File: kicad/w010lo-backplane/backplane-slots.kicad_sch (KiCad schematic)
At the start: 8 parts, among them J3 VME, J4 VME, J5 VME, J6 VME

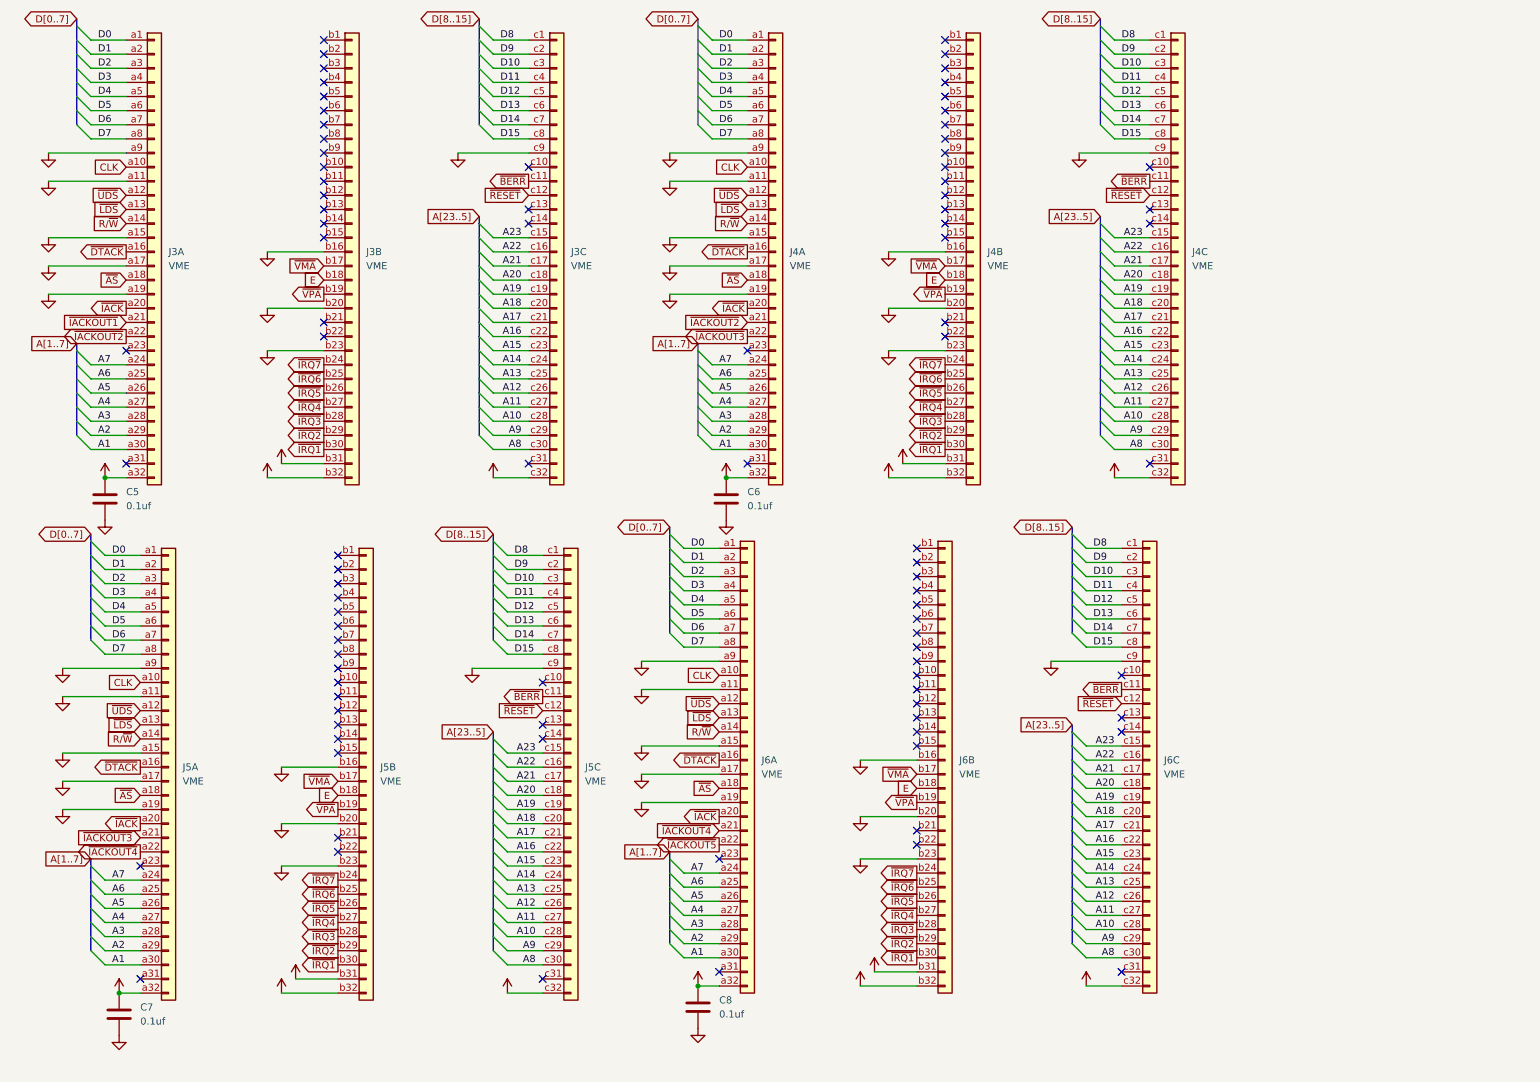
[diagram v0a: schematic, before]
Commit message: Final Kicad update before manufacturing
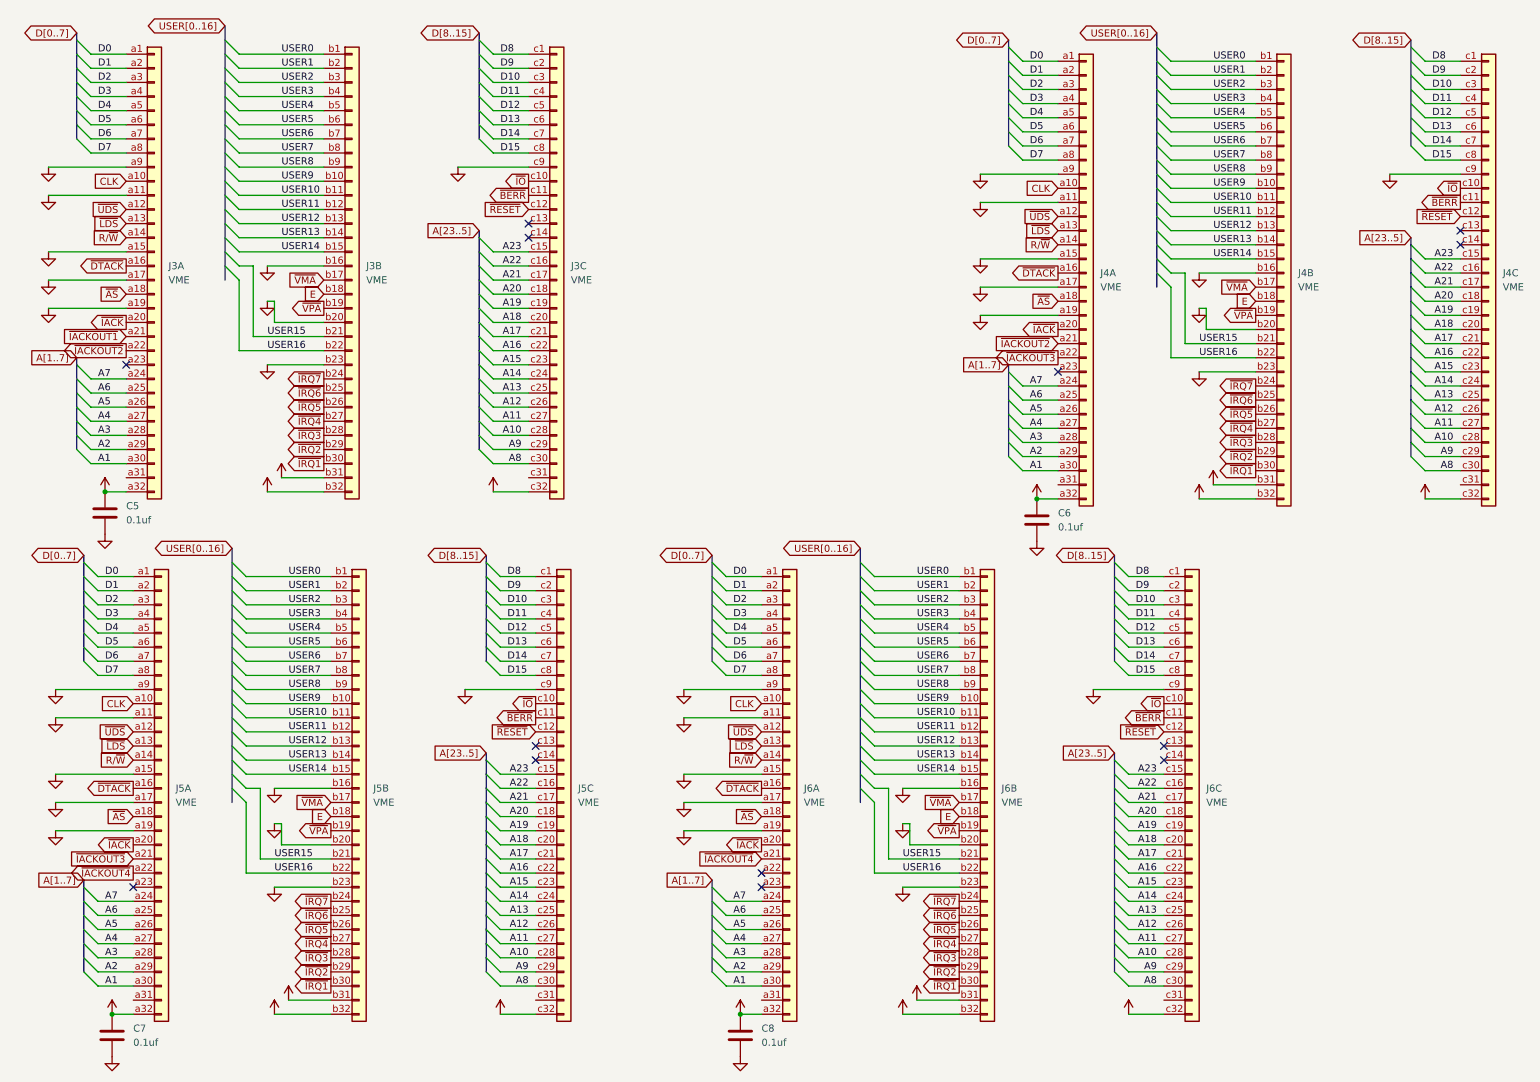
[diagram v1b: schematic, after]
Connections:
- net ~{IO}: now reaches J6.c10 (Pin_c10)
- net ~{IO}: now also J3.c10 (Pin_c10), J4.c10 (Pin_c10), J5.c10 (Pin_c10)
- net USER0: now reaches J6.b1 (Pin_b1)
- net USER0: now also J3.b1 (Pin_b1), J4.b1 (Pin_b1), J5.b1 (Pin_b1)
- net USER9: now reaches J6.b10 (Pin_b10)
- net USER9: now also J3.b10 (Pin_b10), J4.b10 (Pin_b10), J5.b10 (Pin_b10)
- net USER10: now reaches J6.b11 (Pin_b11)
- net USER10: now also J3.b11 (Pin_b11), J4.b11 (Pin_b11), J5.b11 (Pin_b11)
- net USER11: now reaches J6.b12 (Pin_b12)
- net USER11: now also J3.b12 (Pin_b12), J4.b12 (Pin_b12), J5.b12 (Pin_b12)
- net USER12: now reaches J6.b13 (Pin_b13)
- net USER12: now also J3.b13 (Pin_b13), J4.b13 (Pin_b13), J5.b13 (Pin_b13)
- net USER13: now reaches J6.b14 (Pin_b14)
- net USER13: now also J3.b14 (Pin_b14), J4.b14 (Pin_b14), J5.b14 (Pin_b14)
- net USER14: now reaches J6.b15 (Pin_b15)
- net USER14: now also J3.b15 (Pin_b15), J4.b15 (Pin_b15), J5.b15 (Pin_b15)
- net USER1: now reaches J6.b2 (Pin_b2)
- net USER1: now also J3.b2 (Pin_b2), J4.b2 (Pin_b2), J5.b2 (Pin_b2)
- net USER15: now reaches J6.b21 (Pin_b21)
- net USER15: now also J3.b21 (Pin_b21), J4.b21 (Pin_b21), J5.b21 (Pin_b21)
- net USER16: now reaches J6.b22 (Pin_b22)
- net USER16: now also J3.b22 (Pin_b22), J4.b22 (Pin_b22), J5.b22 (Pin_b22)
- net USER2: now reaches J6.b3 (Pin_b3)
- net USER2: now also J3.b3 (Pin_b3), J4.b3 (Pin_b3), J5.b3 (Pin_b3)
- net USER3: now reaches J6.b4 (Pin_b4)
- net USER3: now also J3.b4 (Pin_b4), J4.b4 (Pin_b4), J5.b4 (Pin_b4)
- net USER4: now reaches J6.b5 (Pin_b5)
- net USER4: now also J3.b5 (Pin_b5), J4.b5 (Pin_b5), J5.b5 (Pin_b5)
- net USER5: now reaches J6.b6 (Pin_b6)
- net USER5: now also J3.b6 (Pin_b6), J4.b6 (Pin_b6), J5.b6 (Pin_b6)
- net USER6: now reaches J6.b7 (Pin_b7)
- net USER6: now also J3.b7 (Pin_b7), J4.b7 (Pin_b7), J5.b7 (Pin_b7)
- net USER7: now reaches J6.b8 (Pin_b8)
- net USER7: now also J3.b8 (Pin_b8), J4.b8 (Pin_b8), J5.b8 (Pin_b8)
- net USER8: now reaches J6.b9 (Pin_b9)
- net USER8: now also J3.b9 (Pin_b9), J4.b9 (Pin_b9), J5.b9 (Pin_b9)
- net ~{IACKOUT5}: no longer names the net of J6.a22 (Pin_a22)
- no-connect marks 92 -> 13
